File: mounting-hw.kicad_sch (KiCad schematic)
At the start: 27 parts, among them J1 Conn_01x04, J2 Conn_01x08

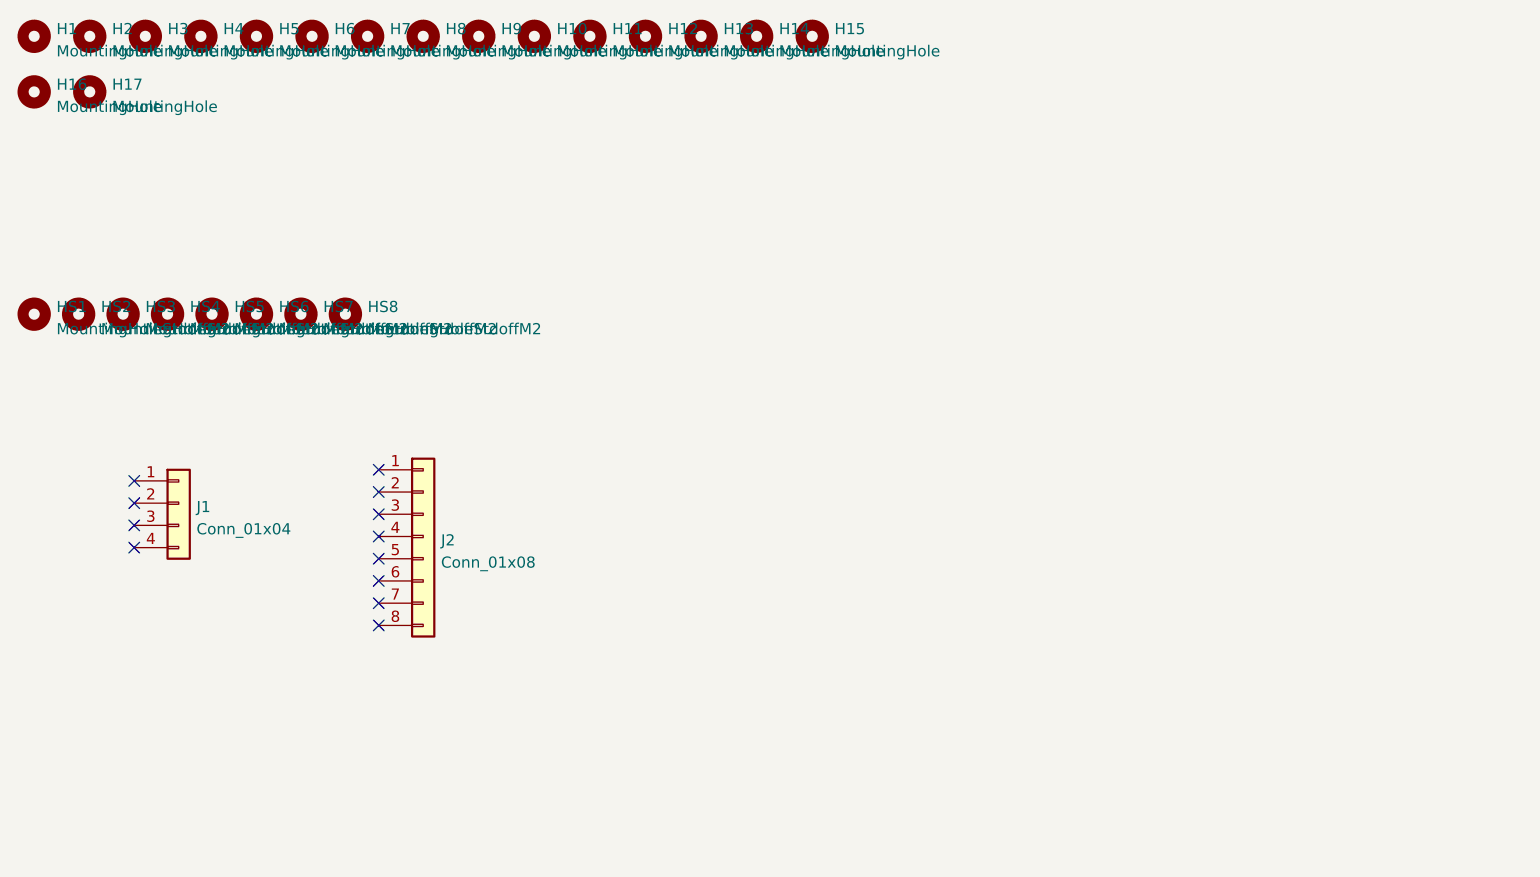
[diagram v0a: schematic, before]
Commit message: More scripts to draw border and place footprint
M  drawborder.py
M  mounting-hw.kicad_sch
M  optical-keyboard-mx.kicad_pcb
M  optical-keyboard-mx.kicad_sch
M  placefp.py
 D placefpg.mx
M  placeholes.py
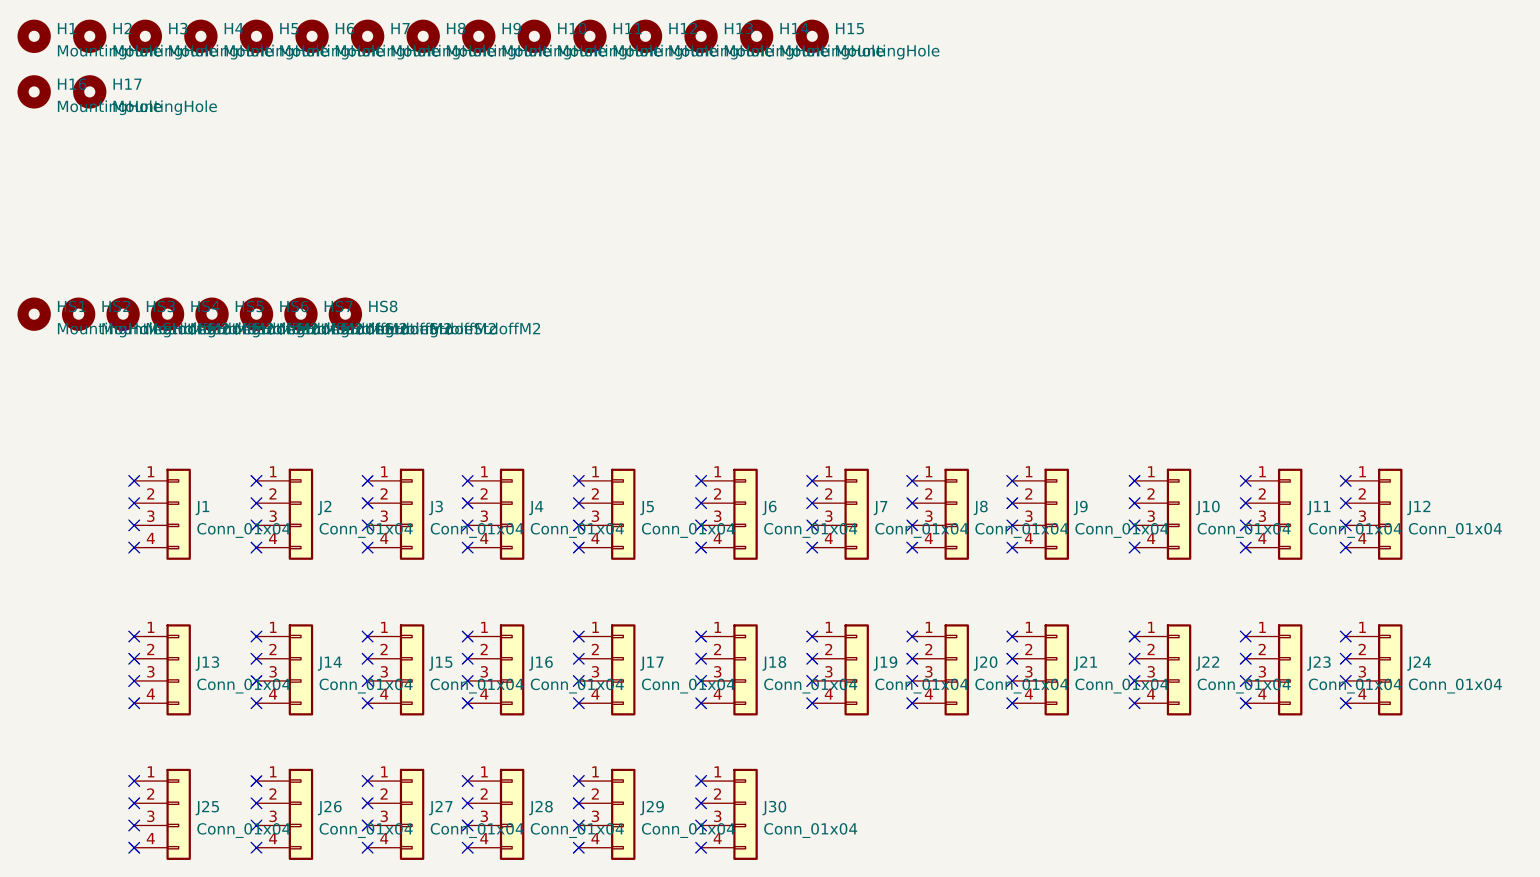
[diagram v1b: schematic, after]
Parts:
- removed J2: Conn_01x08, MyFootprints:PinHeader_1x08_P2.54mm_Vertical, symbol MySymbols:Conn_01x08
- added J10, J11, J12, J13, J14, J15, J16, J17, J18, J19, J2, J20, J21, J22, J23, J24, J25, J26, J27, J28, J29, J3, J30, J4, J5, J6, J7, J8, J9: Conn_01x04, MyFootprints:PinHeader_1x04_P2.54mm_Vertical, symbol MySymbols:Conn_01x04
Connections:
- no-connect marks 12 -> 120
